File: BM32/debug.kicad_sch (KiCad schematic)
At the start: 32 parts, among them J11 Conn_02x05_Odd_Even, J12 Conn_01x03, SW2 SW_Push, U1 BM32F100, U14 SN65HVD7x

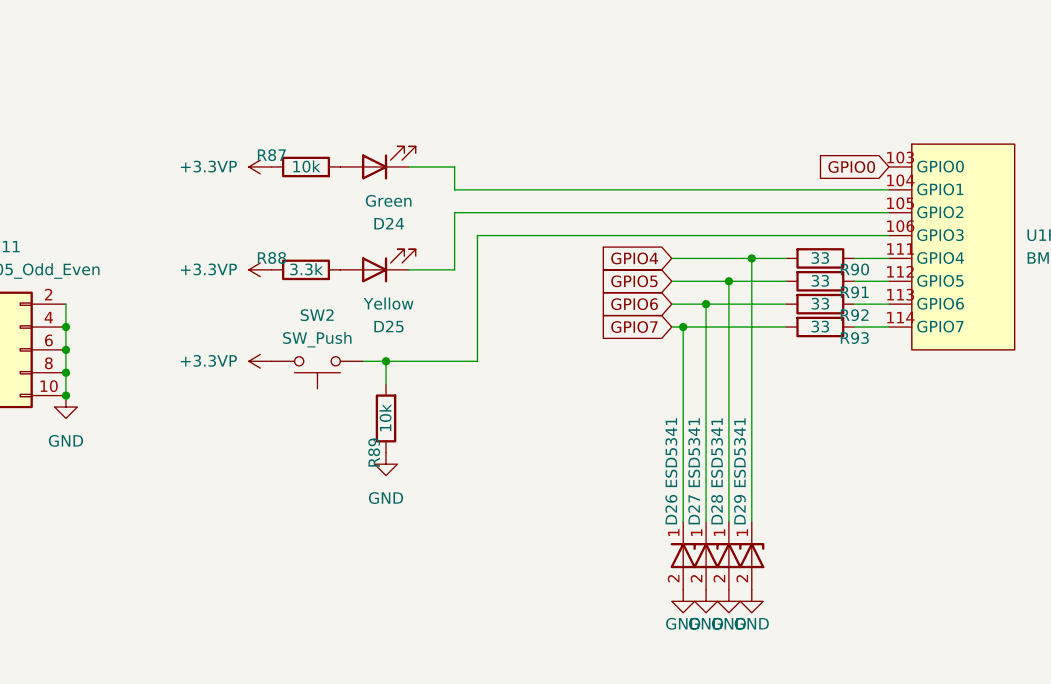
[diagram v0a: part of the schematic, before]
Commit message: Update
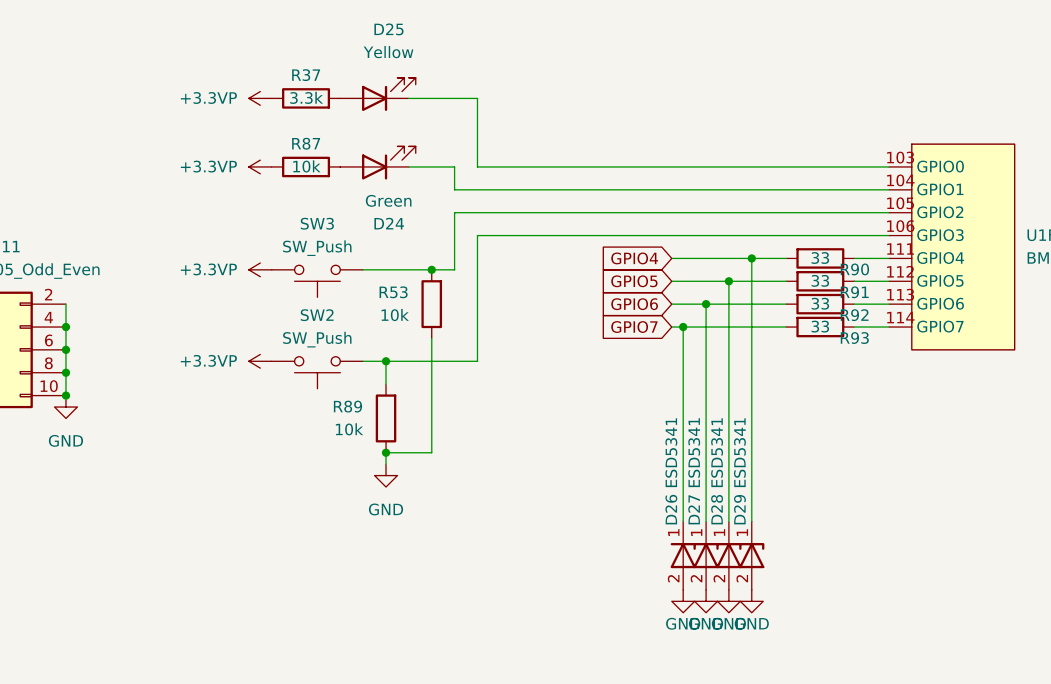
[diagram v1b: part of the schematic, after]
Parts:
- removed R88: 3.3k, lc:0402_R, symbol Device:R
- added R37: 3.3k, lc:0402_R, symbol Device:R
- added R53: 10k, lc:0402_R, symbol Device:R
- added SW3: SW_Push, Button_Switch_SMD:SW_Push_SPST_NO_Alps_SKRK, symbol Switch:SW_Push
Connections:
- net +3.3VP: now also R37.1, SW3.2
- net GND: now also R53.1
- net at D25.2 (A): now also R37.2
- net at U1.105 (GPIO2): now also R53.2, SW3.1; no longer D25.1 (K)
- net GPIO0: no longer names the net of U1.103 (GPIO0)
- net GPIO0: now also D25.1 (K)
